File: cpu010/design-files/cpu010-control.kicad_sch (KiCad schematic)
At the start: 14 parts, among them SW401 SW_DIP_x08, SW402 SW_DIP_x08, U401 DA04-11SURKWA, U402 74HCT273, U403 74HCT273, U404 GAL22V10, U405 74HC245, U406 74HC245, U407 74HCT273, U408 74HC245

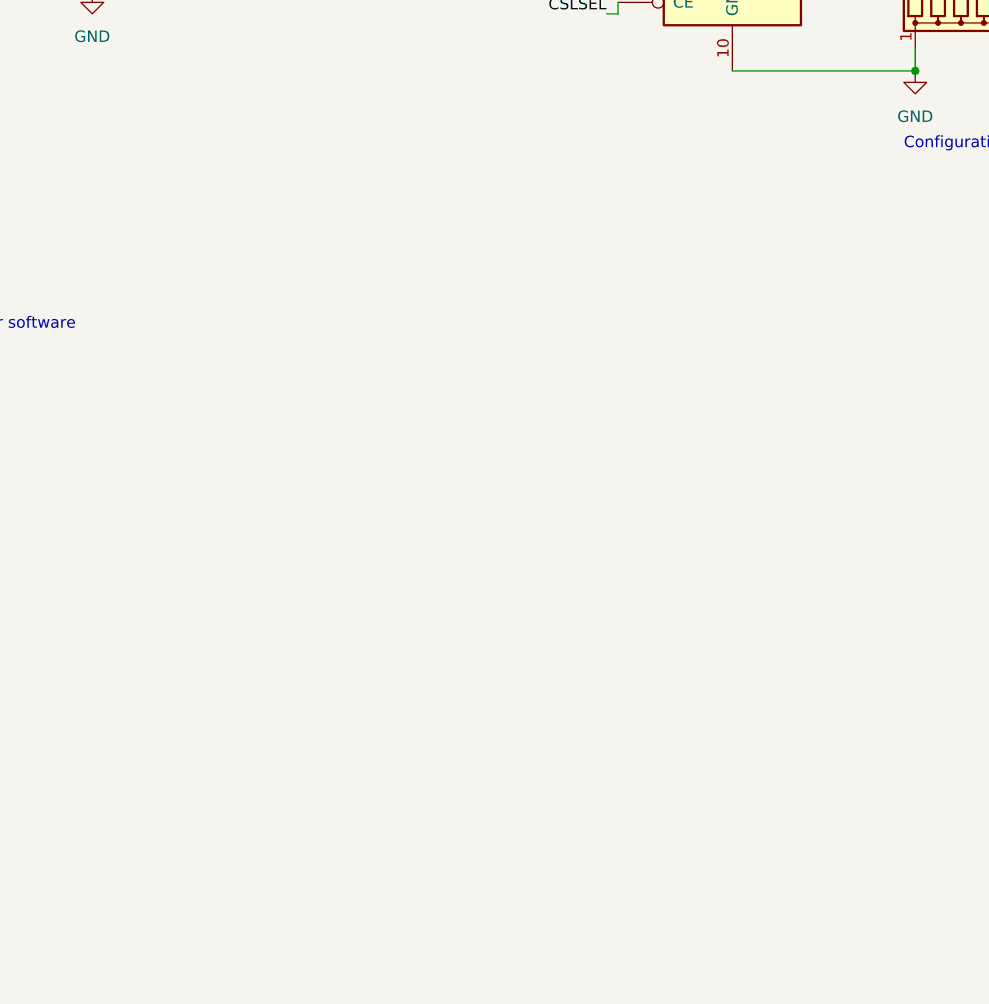
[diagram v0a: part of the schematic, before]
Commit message: Wire up Bus Error register.
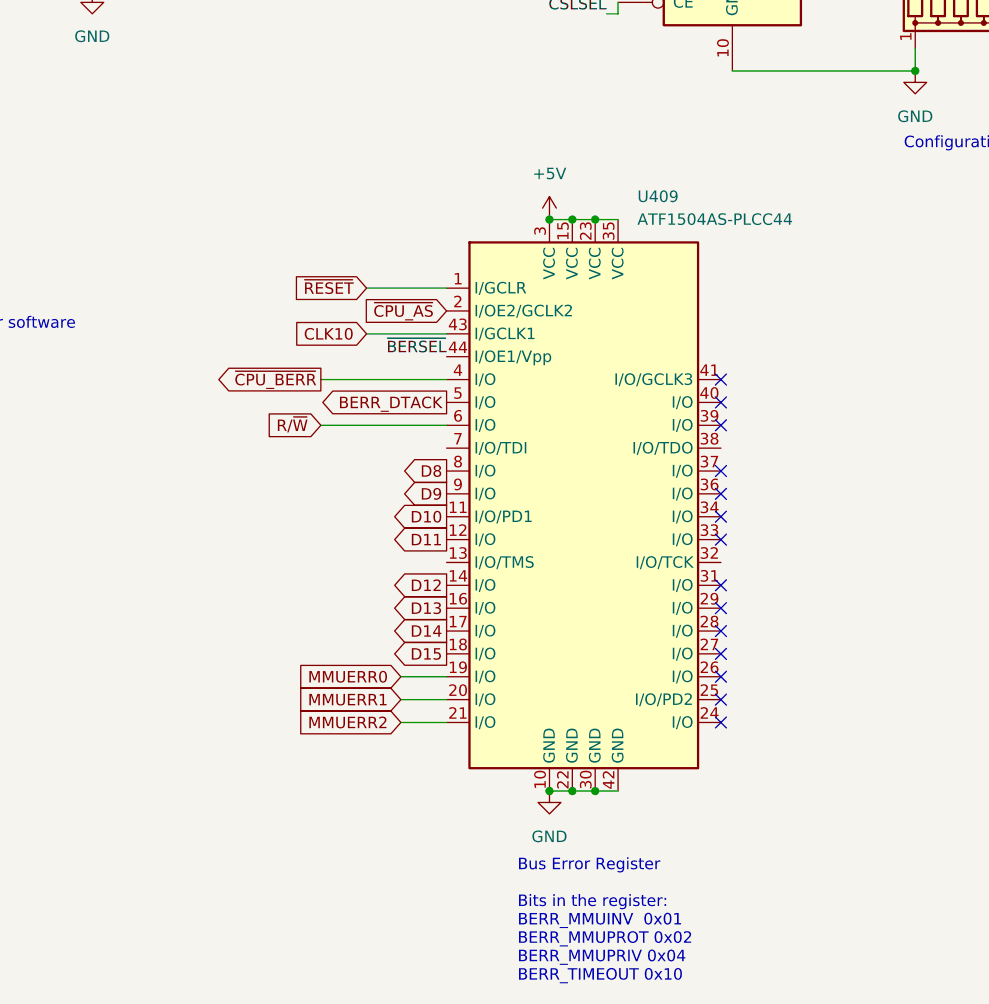
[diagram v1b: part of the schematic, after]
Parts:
- added U409: ATF1504AS-PLCC44, Package_LCC:PLCC-44_THT-Socket, symbol jrt-ICs:ATF1504AS-PLCC44
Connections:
- net +5V: now also U409.15 (VCC), U409.23 (VCC), U409.3 (VCC), U409.35 (VCC)
- net D10: now also U409.11 (I/O/PD1)
- net D11: now also U409.12 (I/O)
- net D12: now also U409.14 (I/O)
- net D13: now also U409.16 (I/O)
- net D14: now also U409.17 (I/O)
- net D15: now also U409.18 (I/O)
- net D8: now also U409.8 (I/O)
- net D9: now also U409.9 (I/O)
- net GND: now also U409.10 (GND), U409.22 (GND), U409.30 (GND), U409.42 (GND)
- net R/~{W}: now also U409.6 (I/O)
- net ~{BERSEL}: now also U409.44 (I/OE1/Vpp)
- net ~{RESET}: now also U409.1 (I/GCLR)
- new net BERR_DTACK: U409.5 (I/O)
- new net CLK10: U409.43 (I/GCLK1)
- new net MMUERR0: U409.19 (I/O)
- new net MMUERR1: U409.20 (I/O)
- new net MMUERR2: U409.21 (I/O)
- new net ~{CPU_AS}: U409.2 (I/OE2/GCLK2)
- new net ~{CPU_BERR}: U409.4 (I/O)
- no-connect marks 10 -> 24
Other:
- note added: "Bus Error Register Bits in the register: BERR_MMUINV 0x01 BERR_MMUPROT 0x02 BERR_MMUPRIV 0x04 BERR_TIMEOUT 0x10"
